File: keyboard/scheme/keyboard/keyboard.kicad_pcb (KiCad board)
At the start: 2 copper layers, 53 parts

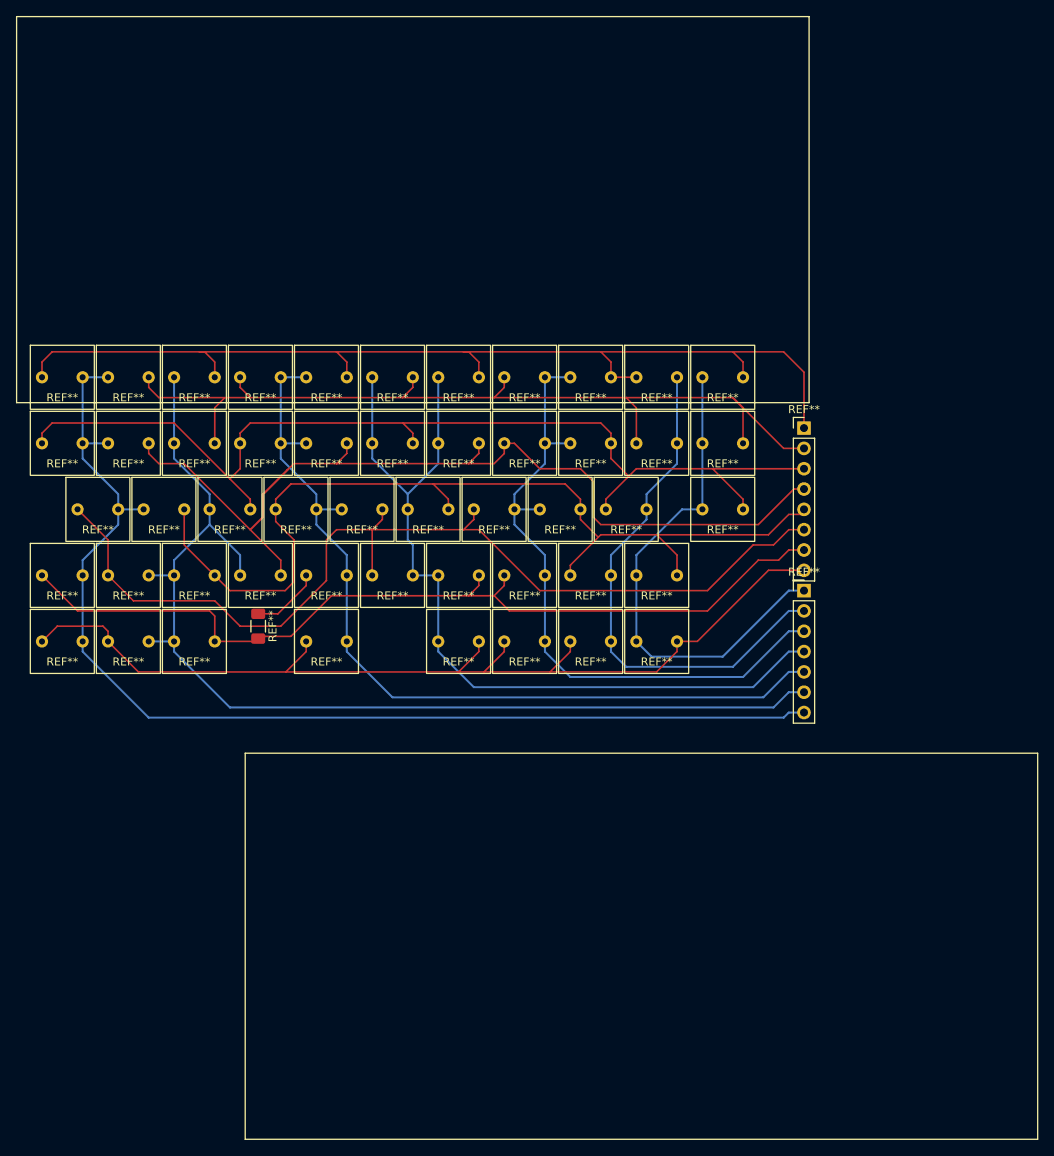
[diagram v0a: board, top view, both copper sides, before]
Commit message: Update keyboard pcd
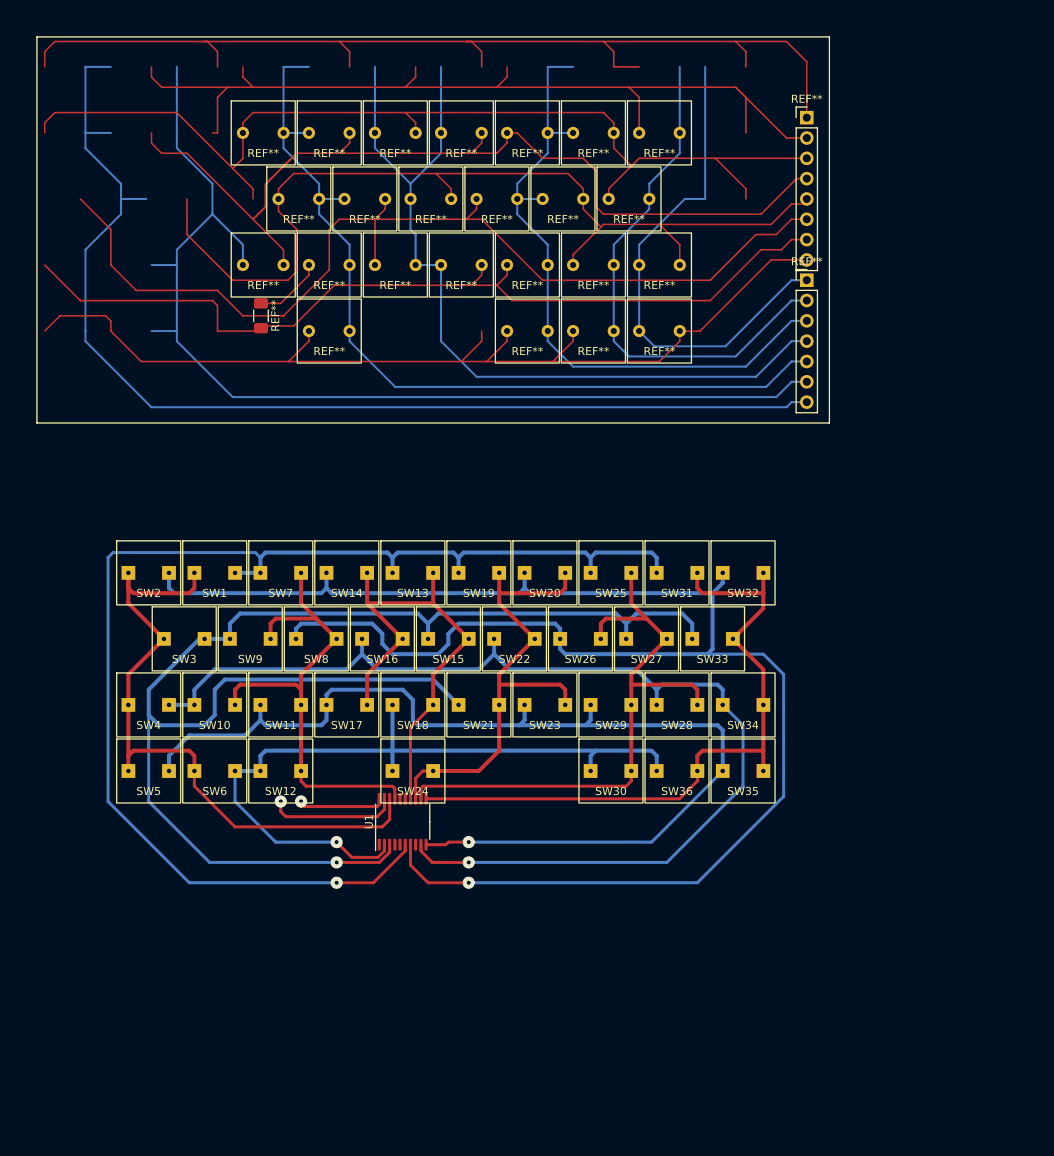
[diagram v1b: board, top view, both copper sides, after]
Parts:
- removed the REF** at (62.9, 64.1)
- removed the REF** at (29.8, 88.9)
- removed the REF** at (79.4, 97.2)
- removed the REF** at (29.8, 64.1)
- removed the REF** at (104.1, 64.1)
- removed the REF** at (95.9, 64.1)
- removed the REF** at (112.4, 80.6)
- removed the REF** at (46.4, 97.2)
- removed the REF** at (71.1, 64.1)
- removed the REF** at (38.1, 64.1)
- removed the REF** at (38.1, 88.9)
- removed the REF** at (38.1, 97.2)
- removed the REF** at (112.4, 72.4)
- removed the REF** at (34.3, 80.6)
- removed the REF** at (46.4, 72.4)
- removed the REF** at (79.4, 64.1)
- removed the REF** at (29.8, 97.2)
- removed the REF** at (46.4, 88.9)
- removed the REF** at (46.4, 64.1)
- removed the REF** at (54.6, 64.1)
- removed the REF** at (87.6, 64.1)
- removed the REF** at (112.4, 64.1)
- removed the REF** at (38.1, 72.4)
- removed the REF** at (29.8, 72.4)
- removed the REF** at (42.5, 80.6)
- removed the REF** at (50.8, 80.6)
- added SW1: SW_DIP_x01, my_lib:btn_8x8, F.Cu at (48.9, 88.6)
- added SW10: SW_DIP_x01, my_lib:btn_8x8, F.Cu at (48.9, 105.1)
- added SW11: SW_DIP_x01, my_lib:btn_8x8, F.Cu at (57.1, 105.1)
- added SW12: SW_DIP_x01, my_lib:btn_8x8, F.Cu at (57.1, 113.3)
- added SW13: SW_DIP_x01, my_lib:btn_8x8, F.Cu at (73.7, 88.6)
- added SW14: SW_DIP_x01, my_lib:btn_8x8, F.Cu at (65.4, 88.6)
- added SW15: SW_DIP_x01, my_lib:btn_8x8, F.Cu at (78.1, 96.8)
- added SW16: SW_DIP_x01, my_lib:btn_8x8, F.Cu at (69.8, 96.8)
- added SW17: SW_DIP_x01, my_lib:btn_8x8, F.Cu at (65.4, 105.1)
- added SW18: SW_DIP_x01, my_lib:btn_8x8, F.Cu at (73.7, 105.1)
- added SW19: SW_DIP_x01, my_lib:btn_8x8, F.Cu at (81.9, 88.6)
- added SW2: SW_DIP_x01, my_lib:btn_8x8, F.Cu at (40.6, 88.6)
- added SW20: SW_DIP_x01, my_lib:btn_8x8, F.Cu at (90.2, 88.6)
- added SW21: SW_DIP_x01, my_lib:btn_8x8, F.Cu at (81.9, 105.1)
- added SW22: SW_DIP_x01, my_lib:btn_8x8, F.Cu at (86.4, 96.8)
- added SW23: SW_DIP_x01, my_lib:btn_8x8, F.Cu at (90.2, 105.1)
- added SW24: SW_DIP_x01, my_lib:btn_8x8, F.Cu at (73.7, 113.3)
- added SW25: SW_DIP_x01, my_lib:btn_8x8, F.Cu at (98.4, 88.6)
- added SW26: SW_DIP_x01, my_lib:btn_8x8, F.Cu at (94.6, 96.8)
- added SW27: SW_DIP_x01, my_lib:btn_8x8, F.Cu at (102.9, 96.8)
- added SW28: SW_DIP_x01, my_lib:btn_8x8, F.Cu at (106.7, 105.1)
- added SW29: SW_DIP_x01, my_lib:btn_8x8, F.Cu at (98.4, 105.1)
- added SW3: SW_DIP_x01, my_lib:btn_8x8, F.Cu at (45.1, 96.8)
- added SW30: SW_DIP_x01, my_lib:btn_8x8, F.Cu at (98.4, 113.3)
- added SW31: SW_DIP_x01, my_lib:btn_8x8, F.Cu at (106.7, 88.6)
- added SW32: SW_DIP_x01, my_lib:btn_8x8, F.Cu at (114.9, 88.6)
- added SW33: SW_DIP_x01, my_lib:btn_8x8, F.Cu at (111.1, 96.8)
- added SW34: SW_DIP_x01, my_lib:btn_8x8, F.Cu at (114.9, 105.1)
- added SW35: SW_DIP_x01, my_lib:btn_8x8, F.Cu at (114.9, 113.3)
- added SW36: SW_DIP_x01, my_lib:btn_8x8, F.Cu at (106.7, 113.3)
- added SW4: SW_DIP_x01, my_lib:btn_8x8, F.Cu at (40.6, 105.1)
- added SW5: SW_DIP_x01, my_lib:btn_8x8, F.Cu at (40.6, 113.3)
- added SW6: SW_DIP_x01, my_lib:btn_8x8, F.Cu at (48.9, 113.3)
- added SW7: SW_DIP_x01, my_lib:btn_8x8, F.Cu at (57.1, 88.6)
- added SW8: SW_DIP_x01, my_lib:btn_8x8, F.Cu at (61.6, 96.8)
- added SW9: SW_DIP_x01, my_lib:btn_8x8, F.Cu at (53.3, 96.8)
- added U1: STM32F030F4Px, Package_SO:TSSOP-20_4.4x6.5mm_P0.65mm, F.Cu at (69.8, 119.7)
- moved REF** 38.8 mm to (71.5, 50.1)
- moved REF** 38.8 mm to (104.5, 50.1)
- moved REF** 38.8 mm to (63.2, 50.1)
- moved REF** 38.8 mm to (79.7, 50.1)
- moved REF** 38.8 mm to (55.0, 50.1)
- moved REF** 38.8 mm to (88.0, 50.1)
- moved REF** 38.8 mm to (96.2, 50.1)
- moved REF** 38.8 mm to (88.0, 58.4)
- moved REF** 38.8 mm to (55.0, 33.6)
- moved REF** 38.8 mm to (104.5, 58.4)
- moved REF** 38.8 mm to (63.2, 58.4)
- moved REF** 38.8 mm to (104.5, 33.6)
- moved REF** 38.8 mm to (79.7, 33.6)
- moved REF** 38.8 mm to (63.2, 33.6)
- moved REF** 38.8 mm to (52.1, 56.5)
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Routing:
- net row_2: track 0.00 -> 227.6 mm, vias 0 -> 1
- net row_3: track 0.00 -> 174.9 mm, vias 0 -> 1
- net row_1: track 0.00 -> 158.2 mm, vias 0 -> 1
- net row_4: track 0.00 -> 141.3 mm, vias 0 -> 1
- net row_5: track 0.00 -> 134.0 mm, vias 0 -> 1
- net row_6: track 0.00 -> 94.6 mm, vias 0 -> 1
- net column_6: track 0.00 -> 84.9 mm
- net column_1: track 0.00 -> 83.1 mm
- net column_5: track 0.00 -> 76.0 mm
- net column_2: track 0.00 -> 61.7 mm
- net column_3: track 0.00 -> 61.6 mm
- net column_4: track 0.00 -> 61.2 mm
- net sw_dio: track 0.00 -> 16.2 mm, vias 0 -> 1
- net sw_clk: track 0.00 -> 11.2 mm, vias 0 -> 1
